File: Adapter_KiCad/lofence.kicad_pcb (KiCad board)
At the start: 2 copper layers, 78 x 130 mm, 25 parts, among them J1 Fence+, J2 Fence-, U1 Opamp_Dual_Generic, U2 WIFI_KIT_32__V3_

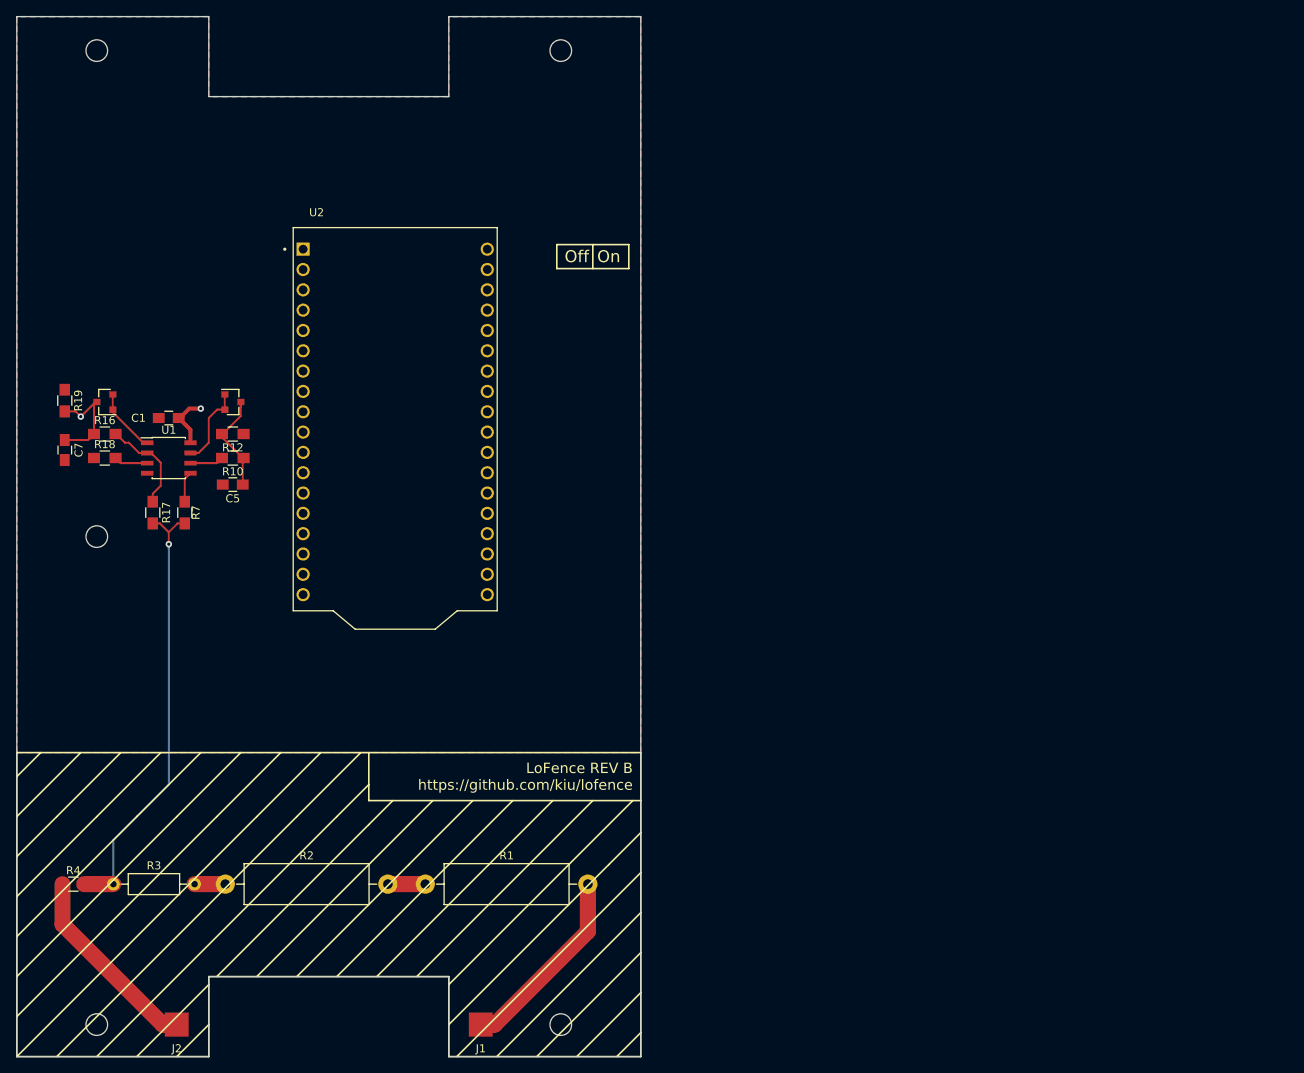
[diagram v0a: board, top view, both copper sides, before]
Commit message: Finished PCB & Schematic
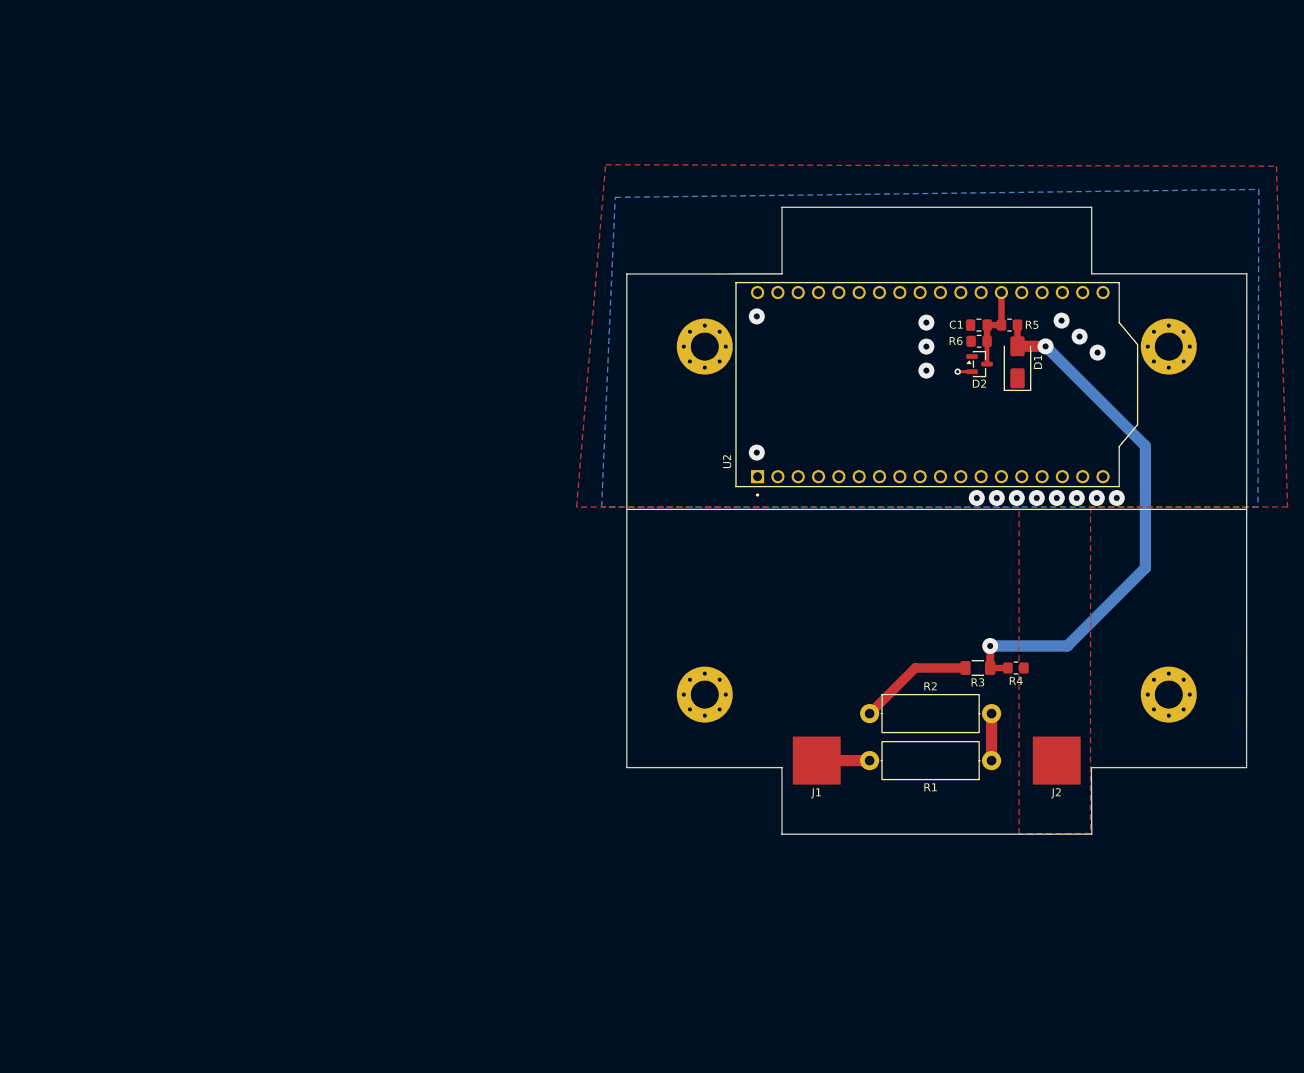
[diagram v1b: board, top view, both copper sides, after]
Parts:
- removed C5, C7: 100nF, Capacitors_SMD:C_0805_HandSoldering
- removed D8: BAV70LT, TO_SOT_Packages_SMD:SOT-23
- removed MH1, MH3, MH4, MH5, MH6: MountingHole, Mounting_Holes:MountingHole_2.7mm_M2.5
- removed R10, R16, R17, R18, R7: 100k, Resistors_SMD:R_0805_HandSoldering
- removed R12, R19: 1M, Resistors_SMD:R_0805_HandSoldering
- removed U1: Opamp_Dual_Generic, Housings_SOIC:SOIC-8_3.9x4.9mm_Pitch1.27mm
- added D1: SMAJ5.0CA, Diode_SMD:D_SMA, F.Cu at (160.1, 80.2)
- added R5: 10k, Resistor_SMD:R_0805_2012Metric_Pad1.20x1.40mm_HandSolder, F.Cu at (159.1, 75.6)
- added R6: 1M, Resistor_SMD:R_0805_2012Metric_Pad1.20x1.40mm_HandSolder, F.Cu at (155.3, 77.6)
- added REF**: MountingHole_3.5mm_Pad_Via, MountingHole:MountingHole_3.5mm_Pad_Via, F.Cu at (121.0, 121.8)
- added REF**: MountingHole_3.5mm_Pad_Via, MountingHole:MountingHole_3.5mm_Pad_Via, F.Cu at (179.0, 121.8)
- added REF**: MountingHole_3.5mm_Pad_Via, MountingHole:MountingHole_3.5mm_Pad_Via, F.Cu at (121.0, 78.2)
- added REF**: MountingHole_3.5mm_Pad_Via, MountingHole:MountingHole_3.5mm_Pad_Via, F.Cu at (179.0, 78.2)
- C1: footprint Capacitors_SMD:C_0805_HandSoldering -> Capacitor_SMD:C_0805_2012Metric_Pad1.18x1.45mm_HandSolder
- D2: value BAV70LT -> BAT54S; footprint TO_SOT_Packages_SMD:SOT-23 -> Package_TO_SOT_SMD:SOT-23
- R1, R2: footprint Resistors_ThroughHole:R_Axial_DIN0516_L15.5mm_D5.0mm_P20.32mm_Horizontal -> Resistor_THT:R_Axial_DIN0414_L11.9mm_D4.5mm_P15.24mm_Horizontal
- R3: footprint Resistors_ThroughHole:R_Axial_DIN0207_L6.3mm_D2.5mm_P10.16mm_Horizontal -> Resistor_SMD:R_1206_3216Metric_Pad1.30x1.75mm_HandSolder
- R4: value 5k8 -> 5k1; footprint Resistors_SMD:R_0805_HandSoldering -> Resistor_SMD:R_0805_2012Metric_Pad1.20x1.40mm_HandSolder
- moved R4 120.9 mm to (159.9, 118.4), turned to 180 degrees
- moved J2 114.8 mm to (165.0, 130.0)
- moved R3 111.4 mm to (155.1, 118.4), turned to 180 degrees
- moved C1 101.9 mm to (155.3, 75.6)
- moved D2 93.5 mm to (155.3, 80.4)
- moved R2 83.3 mm to (141.6, 124.1)
- moved R1 72.4 mm to (156.8, 130.0), turned to 180 degrees
- moved U2 67.9 mm to (150.0, 83.0), turned to 90 degrees
- moved J1 53.4 mm to (135.0, 130.0)
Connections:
- net PROBE renamed Net-(D1-A2)
- C1 pad 1: ADC_POWER -> ADC_FENCE
- D2 pad 1: Net-(D2-A1) -> GND
- D2 pad 2: Net-(D2-A1) -> +3.3V
- D2 pad 3: ADC+ -> ADC_FENCE
- U2 pad J2_1: unconnected-(U2A-GND_J2-PadJ2_1) -> GND
- U2 pad J2_2: unconnected-(U2A-5V-PadJ2_2) -> +5V
- U2 pad J2_3: VE -> unconnected-(U2A-VE/OUTPUT_3.3V-PadJ2_3)
- U2 pad J2_4: VE -> unconnected-(U2A-VE/OUTPUT_3.3V-PadJ2_4)
- U2 pad J3_1: unconnected-(U2B-GND_J3-PadJ3_1) -> GND
- U2 pad J3_13: unconnected-(U2B-GPIO39/MTCK-PadJ3_13) -> ADC_FENCE
- U2 pad J3_2: 3V3 -> +3.3V
- U2 pad J3_3: 3V3 -> +3.3V
- U2 pad J3_4: unconnected-(U2B-GPIO26/SPICS1-PadJ3_4) -> +3.3V
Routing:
- net GND: track 24.5 -> 0.00 mm, vias 0 -> 16
- net Net-(J1-Pin_1): track 24.1 -> 6.60 mm
- net ADC-: track 13.1 -> 0.00 mm, vias 1 -> 0
- net ADC+: track 12.6 -> 0.00 mm
- net Net-(U1A--): track 12.4 -> 0.00 mm
- net Net-(D1-A2): track 55.9 -> 67.5 mm, vias 1 -> 2
- net ADC_FENCE: track 0.00 -> 10.7 mm
- net Net-(R2-Pad1): track 3.84 -> 14.3 mm
- net Net-(D2-A1): track 10.3 -> 0.00 mm
- net Net-(D8-A1): track 8.10 -> 0.00 mm
- net ADC_POWER: track 6.93 -> 0.00 mm, vias 1 -> 0
- net Net-(U1B--): track 4.21 -> 0.00 mm
- net Net-(U1A-+): track 4.21 -> 0.00 mm
- net Net-(U1B-+): track 3.85 -> 0.00 mm
- net +3.3V: track 0.00 -> 1.79 mm, vias 0 -> 1
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- added copper zone on In1.Cu, net +3.3V
- added copper zone on In2.Cu, net GND
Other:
- board size 78 x 130 mm -> 77.5 x 78.4 mm
- copper layers 2 -> 4
- board text removed: "LoFence REV B https://github.com/kiu/lofence"
- board text removed: "Off"
- board text removed: "On"
